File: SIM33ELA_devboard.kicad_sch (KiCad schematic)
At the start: 12 parts, among them J2 Conn_01x13_Pin, U2 SIM33ELA

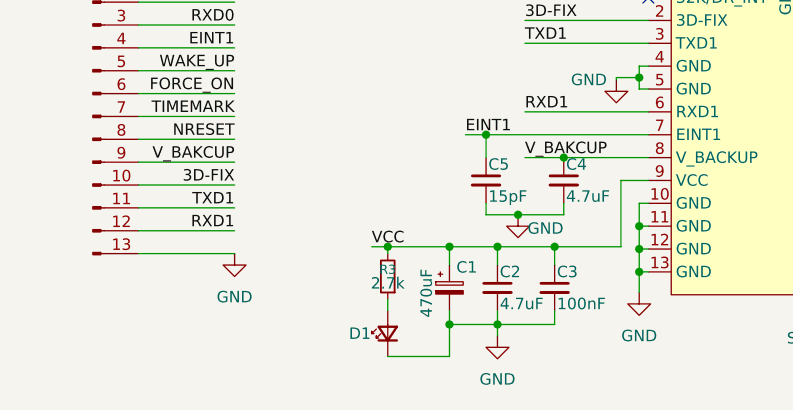
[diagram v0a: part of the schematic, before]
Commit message: por si acaso
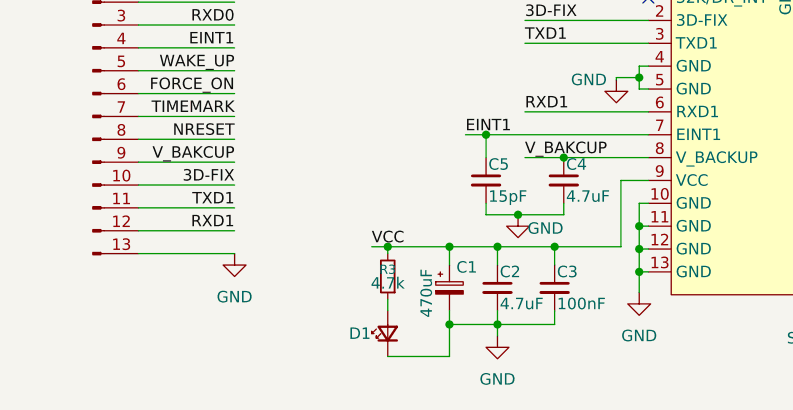
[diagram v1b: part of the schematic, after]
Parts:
- R3: value 2.7k -> 4.7k
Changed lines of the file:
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@@
 			)
 		)
-		(property "Value" "2.7k"
+		(property "Value" "4.7k"
 			(at 114.3 119.634 0)
 			(effects

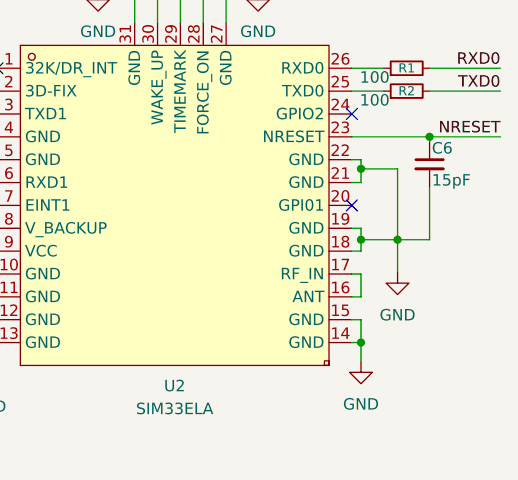
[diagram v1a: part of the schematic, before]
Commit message: cambios finales
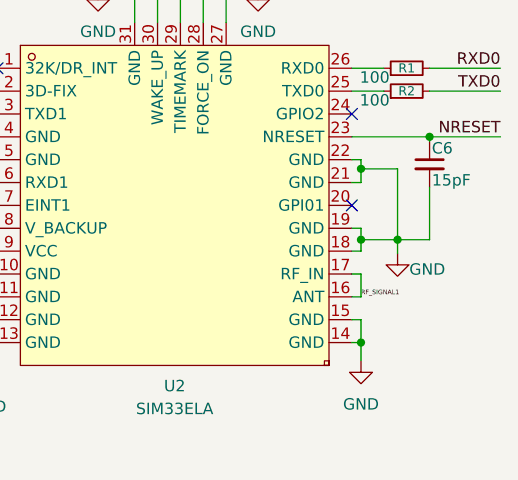
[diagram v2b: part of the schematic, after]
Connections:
- net RF_SIGNAL1: now reaches U2.16 (ANT), U2.17 (RF_IN)
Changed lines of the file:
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@@
+	(wire
+		(pts
+			(xy 183.642 110.744) (xy 183.642 113.284)
+		)
+		(stroke
+			(width 0)
+			(type default)
+		)
+	)
+	(wire
+		(pts
+			(xy 183.642 113.284) (xy 182.626 113.284)
+		)
+		(stroke
+			(width 0)
+			(type default)
+		)
+	)
 	(wire
 		(pts
@@
 	(wire
 		(pts
-			(xy 187.706 110.49) (xy 187.706 106.934)
+			(xy 187.706 108.458) (xy 187.706 106.934)
 		)
 		(stroke
@@
 	(wire
 		(pts
-			(xy 183.642 110.744) (xy 183.642 113.284)
-		)
-		(stroke
-			(width 0)
-			(type default)
-		)
-	)
-	(wire
-		(pts
 			(xy 183.642 115.824) (xy 183.642 118.364)
 		)
@@
 		(pts
 			(xy 142.24 113.284) (xy 143.256 113.284)
-		)
-		(stroke
-			(width 0)
-			(type default)
-		)
-	)
-	(wire
-		(pts
-			(xy 183.642 113.284) (xy 182.626 113.284)
 		)
 		(stroke
@@
 			(font
 				(size 1.27 1.27)
+			)
+			(justify left bottom)
+		)
+	)
+	(label "RF_SIGNAL1"
+		(at 183.642 113.284 0)
+		(effects
+			(font
+				(size 0.508 0.508)
 			)
 			(justify left bottom)
@@
 	(symbol
 		(lib_id "power:GND")
-		(at 187.706 110.49 0)
+		(at 187.706 108.458 0)
 		(unit 1)
 		(exclude_from_sim no)
@@
 		(on_board yes)
 		(dnp no)
-		(fields_autoplaced yes)
 		(property "Reference" "#PWR03"
-			(at 187.706 116.84 0)
+			(at 187.706 114.808 0)
 			(effects
 				(font
@@
 		)
 		(property "Value" "GND"
-			(at 187.706 115.316 0)
+			(at 191.008 110.236 0)
 			(effects
 				(font
@@
 		)
 		(property "Footprint" ""
-			(at 187.706 110.49 0)
+			(at 187.706 108.458 0)
 			(effects
 				(font
@@
 		)
 		(property "Datasheet" ""
-			(at 187.706 110.49 0)
+			(at 187.706 108.458 0)
 			(effects
 				(font
@@
 		)
 		(property "Description" "Power symbol creates a global label with name \"GND\" , ground"
-			(at 187.706 110.49 0)
-			(effects
-				(font
+			(at 187.706 108.458 0)
+			(effects
+				(font

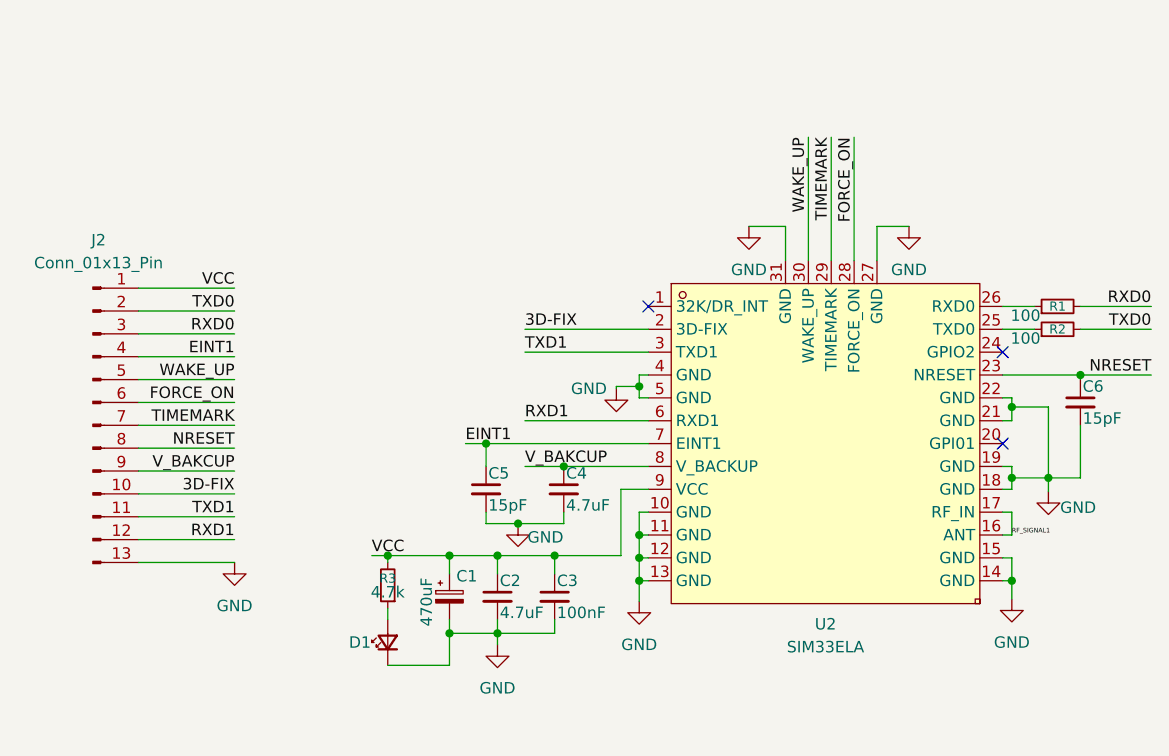
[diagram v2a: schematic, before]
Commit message: aaa
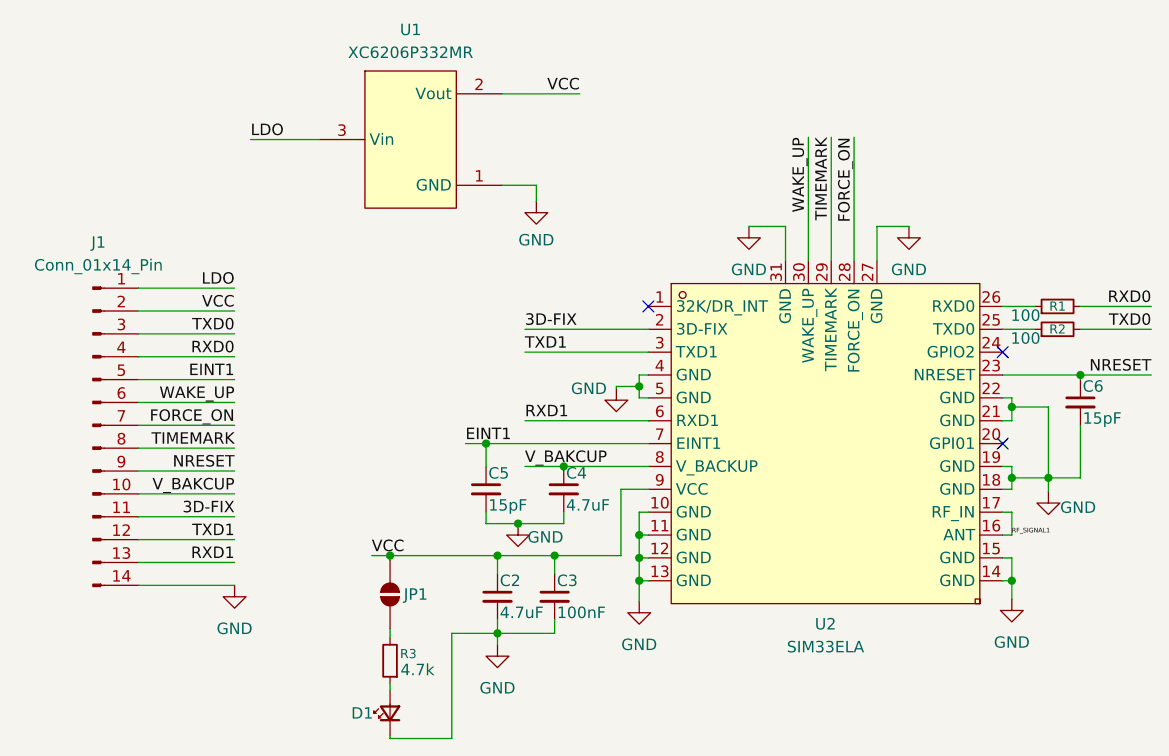
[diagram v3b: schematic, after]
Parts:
- removed C1: 470uF, Capacitor_SMD:CP_Elec_6.3x7.7, symbol Device:C_Polarized_Small
- removed J2: Conn_01x13_Pin, Connector_PinHeader_2.54mm:PinHeader_1x13_P2.54mm_Vertical, symbol Connector:Conn_01x13_Pin
- added J1: Conn_01x14_Pin, Connector_PinHeader_2.54mm:PinHeader_1x14_P2.54mm_Vertical, symbol Connector:Conn_01x14_Pin
- added JP1: SolderJumper_2_Open, Jumper:SolderJumper-2_P1.3mm_Open_RoundedPad1.0x1.5mm, symbol Jumper:SolderJumper_2_Open
- added U1: XC6206P332MR, EasyEDA:SOT-23-3_L2.9-W1.6-P1.90-LS2.8-BR, symbol EasyEDA:XC6206P332MR
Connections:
- net 3D-FIX: now also J1.11 (Pin_11)
- net EINT1: now also J1.5 (Pin_5)
- net FORCE_ON: now also J1.7 (Pin_7)
- net GND: now also J1.14 (Pin_14), U1.1 (GND)
- net NRESET: now also J1.9 (Pin_9)
- net RXD0: now also J1.4 (Pin_4)
- net RXD1: now also J1.13 (Pin_13)
- net TIMEMARK: now also J1.8 (Pin_8)
- net TXD0: now also J1.3 (Pin_3)
- net TXD1: now also J1.12 (Pin_12)
- net VCC: now also J1.2 (Pin_2), JP1.2 (B), U1.2 (Vout); no longer R3.2
- net V_BAKCUP: now also J1.10 (Pin_10)
- net WAKE_UP: now also J1.6 (Pin_6)
- new net: JP1.1 (A), R3.2
- new net LDO: J1.1 (Pin_1), U1.3 (Vin)
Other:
- moved on the sheet: D1, R3
